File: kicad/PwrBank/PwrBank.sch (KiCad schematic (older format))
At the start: 6 parts

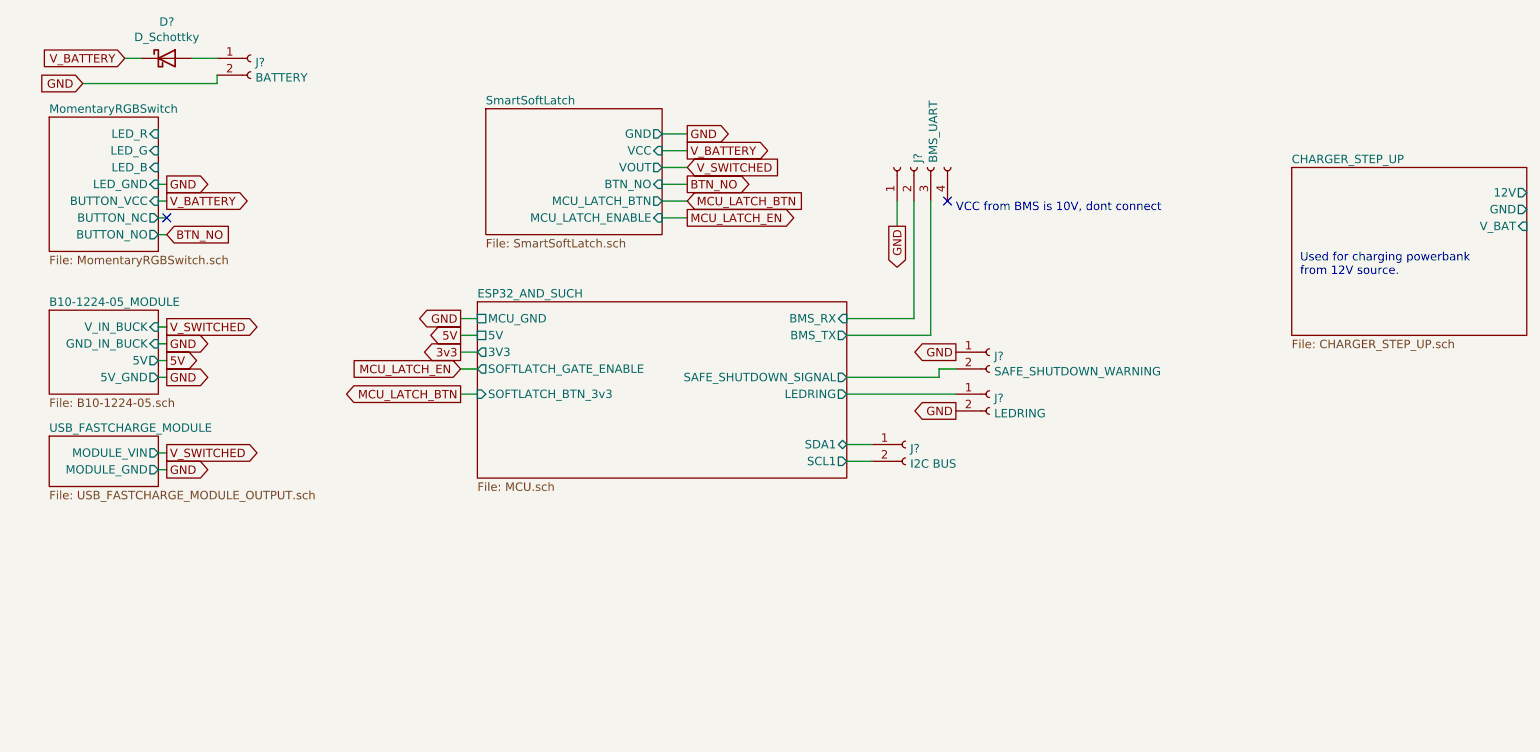
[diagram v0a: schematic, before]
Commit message: UPDATE KICAD SOURCEFILES
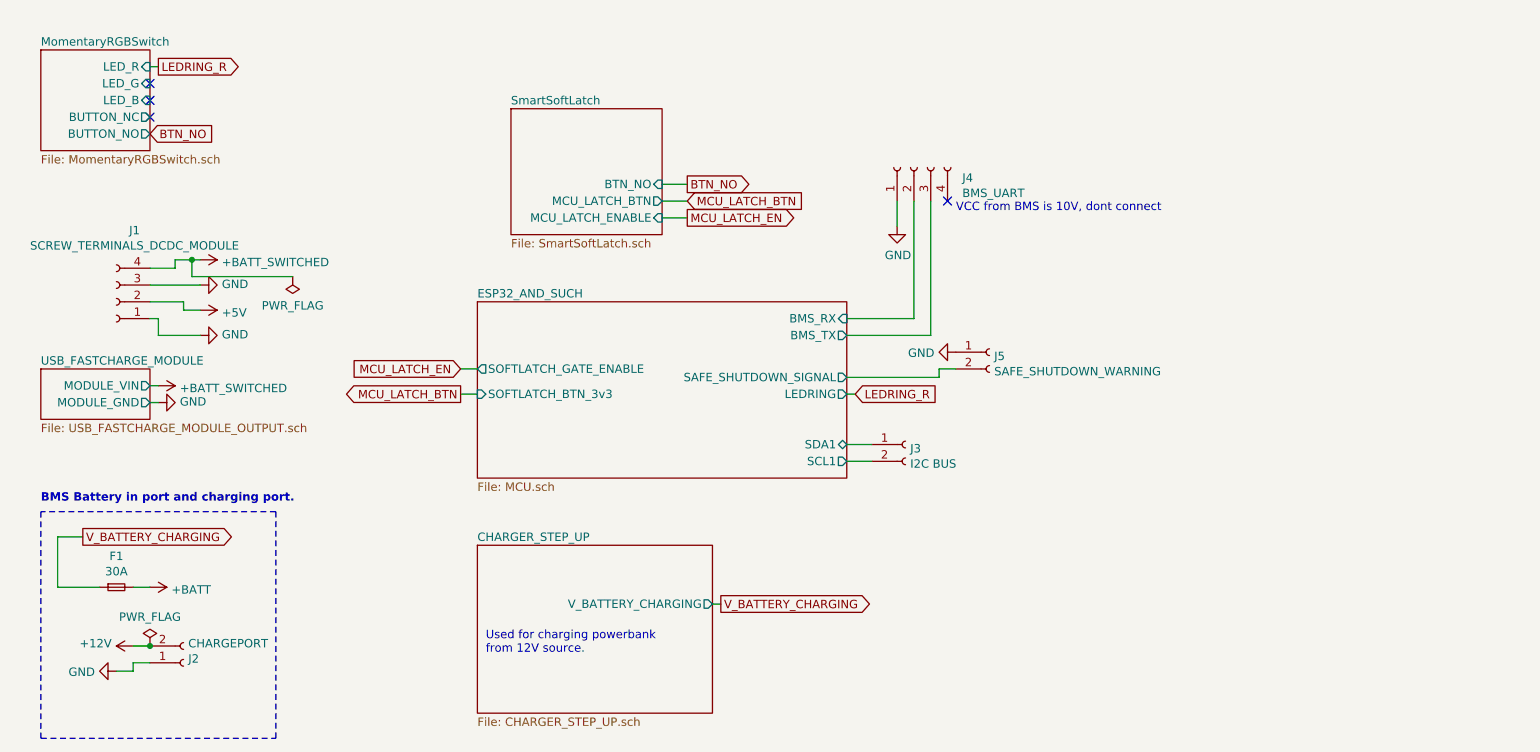
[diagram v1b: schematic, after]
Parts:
- removed D?: D_Schottky, symbol Device:D_Schottky
- removed J?: LEDRING, symbol Connector:Conn_01x02_Female
- removed J?: BATTERY, symbol Connector:Conn_01x02_Female
- added F1: 30A, Fuse:Fuseholder_Blade_Mini_Keystone_3568, symbol Device:Fuse_Small
- added J1: SCREW_TERMINALS_DCDC_MODULE, symbol Connector:Conn_01x04_Female
- added J2: CHARGEPORT, Connector_JST:JST_XH_B2B-XH-A_1x02_P2.50mm_Vertical, symbol Connector:Conn_01x02_Female
- J3, J5: renamed from J?; footprint (none) -> Connector_JST:JST_XH_B2B-XH-A_1x02_P2.50mm_Vertical
- J4: renamed from J?; footprint (none) -> Connector_JST:JST_XH_B4B-XH-A_1x04_P2.50mm_Vertical
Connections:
- net GND: now also J1.1 (Pin_1), J1.3 (Pin_3), J2.1 (Pin_1)
- new net +12V: J2.2 (Pin_2)
- new net +5V: J1.2 (Pin_2)
- new net +BATT: F1.2
- new net +BATT_SWITCHED: J1.4 (Pin_4)
- new net V_BATTERY_CHARGING: F1.1
- no-connect marks 2 -> 4
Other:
- note added: "BMS Battery in port and charging port."

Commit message: Kicad files update
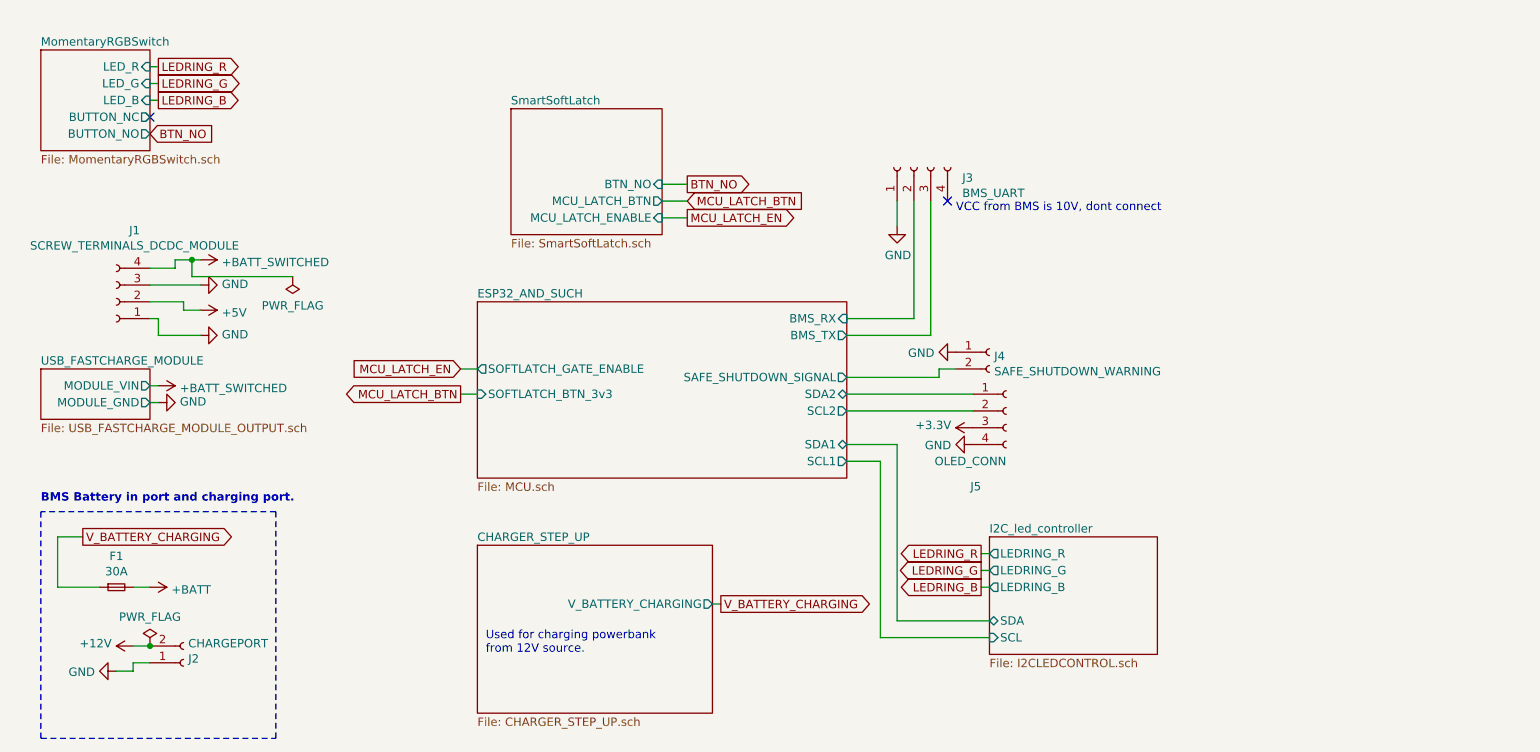
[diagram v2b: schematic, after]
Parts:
- removed J3: I2C BUS, Connector_JST:JST_XH_B2B-XH-A_1x02_P2.50mm_Vertical, symbol Connector:Conn_01x02_Female
- added J5: OLED_CONN, Connector_JST:JST_XH_B4B-XH-A_1x04_P2.50mm_Vertical, symbol Connector:Conn_01x04_Female
- renumbered J4 to J3, J5 to J4
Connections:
- net GND: now also J5.4 (Pin_4)
- new net +3V3: J5.3 (Pin_3)
- new net ESP32_AND_SUCH/SCL2: J5.2 (Pin_2)
- new net ESP32_AND_SUCH/SDA2: J5.1 (Pin_1)
- no-connect marks 4 -> 2
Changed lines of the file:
@@
 $Descr A4 11693 8268
 encoding utf-8
-Sheet 1 8
+Sheet 1 9
 Title "Powerbank BMS Additional Circuitry"
 Date "2021-07-11"
@@
 F3 "LED_G" I R 1250 900 50
 F4 "LED_B" I R 1250 1000 50
-F7 "BUTTON_NC" O R 1250 1100 50
-F8 "BUTTON_NO" O R 1250 1200 50
+F5 "BUTTON_NC" O R 1250 1100 50
+F6 "BUTTON_NO" O R 1250 1200 50
 $EndSheet
 NoConn ~ 1250 1100
@@
 F0 "SmartSoftLatch" 50
 F1 "SmartSoftLatch.sch" 50
-F3 "BTN_NO" I R 4300 1500 50
-F5 "MCU_LATCH_BTN" O R 4300 1600 50
-F6 "MCU_LATCH_ENABLE" I R 4300 1700 50
+F2 "BTN_NO" I R 4300 1500 50
+F3 "MCU_LATCH_BTN" O R 4300 1600 50
+F4 "MCU_LATCH_ENABLE" I R 4300 1700 50
 $EndSheet
 Text GLabel 4450 1500 2    50   Output ~ 0
@@
 F0 "CHARGER_STEP_UP" 50
 F1 "CHARGER_STEP_UP.sch" 50
-F3 "V_BATTERY_CHARGING" O R 4600 4000 50
+F2 "V_BATTERY_CHARGING" O R 4600 4000 50
 $EndSheet
 Text Notes 3250 4300 0    50   ~ 0
@@
 F4 "SAFE_SHUTDOWN_SIGNAL" O R 5400 2650 50
 F5 "SOFTLATCH_GATE_ENABLE" O L 3200 2600 50
-F6 "LEDRING" O R 5400 2750 50
-F7 "SDA1" B R 5400 3050 50
-F8 "SCL1" O R 5400 3150 50
-F9 "SOFTLATCH_BTN_3v3" I L 3200 2750 50
+F6 "SDA1" B R 5400 3050 50
+F7 "SCL1" O R 5400 3150 50
+F8 "SOFTLATCH_BTN_3v3" I L 3200 2750 50
+F9 "SCL2" O R 5400 2850 50
+F10 "SDA2" B R 5400 2750 50
 $EndSheet
 Text GLabel 3100 2600 0    50   Input ~ 0
@@
 Text GLabel 4450 1600 2    50   Input ~ 0
 MCU_LATCH_BTN
-$Comp
-L Connector:Conn_01x02_Female J3
-U 1 1 60F61784
-P 5750 3050
-F 0 "J3" H 5778 3026 50  0000 L CNN
-F 1 "I2C BUS" H 5778 2935 50  0000 L CNN
-F 2 "Connector_JST:JST_XH_B2B-XH-A_1x02_P2.50mm_Vertical" H 5750 3050 50  0001 C CNN
-F 3 "~" H 5750 3050 50  0001 C CNN
-	1    5750 3050
-	1    0    0    -1
-$EndComp
-Wire Wire Line
-	5400 3050 5550 3050
-Wire Wire Line
-	5550 3150 5400 3150
 Wire Wire Line
 	5400 2650 5950 2650
@@
 	5950 2600 6050 2600
 $Comp
-L Connector:Conn_01x04_Female J4
+L Connector:Conn_01x04_Female J3
 U 1 1 60F67167
 P 5800 1400
-F 0 "J4" V 5738 1112 50  0000 R CNN
+F 0 "J3" V 5738 1112 50  0000 R CNN
 F 1 "BMS_UART" V 5647 1112 50  0000 R CNN
 F 2 "Connector_JST:JST_XH_B4B-XH-A_1x04_P2.50mm_Vertical" H 5800 1400 50  0001 C CNN
@@
 Text Notes 600  3400 0    50   ~ 10
 BMS Battery in port and charging port.
-Text GLabel 5450 2750 2    50   Input ~ 0
-LEDRING_R
-Wire Wire Line
-	5450 2750 5400 2750
 Text GLabel 1300 800  2    50   Output ~ 0
 LEDRING_R
 Wire Wire Line
 	1300 800  1250 800
-NoConn ~ 1250 900
-NoConn ~ 1250 1000
 $Comp
 L power:+BATT #PWR03
@@
 $EndComp
 $Comp
-L Connector:Conn_01x02_Female J5
+L Connector:Conn_01x02_Female J4
 U 1 1 60F64EEF
 P 6250 2500
-F 0 "J5" H 6278 2476 50  0000 L CNN
+F 0 "J4" H 6278 2476 50  0000 L CNN
 F 1 "SAFE_SHUTDOWN_WARNING" H 6278 2385 50  0000 L CNN
 F 2 "Connector_JST:JST_XH_B2B-XH-A_1x02_P2.50mm_Vertical" H 6250 2500 50  0001 C CNN
@@
 	0    1    1    0
 $EndComp
+$Comp
+L Connector:Conn_01x04_Female J5
+U 1 1 60F9EBFE
+P 6350 2850
+F 0 "J5" H 6200 2400 50  0000 R CNN
+F 1 "OLED_CONN" H 6350 2550 50  0000 R CNN
+F 2 "Connector_JST:JST_XH_B4B-XH-A_1x04_P2.50mm_Vertical" H 6350 2850 50  0001 C CNN
+F 3 "https://www.jst-mfg.com/product/pdf/eng/eXH.pdf" H 6350 2850 50  0001 C CNN
+	1    6350 2850
+	1    0    0    -1
+$EndComp
+Wire Wire Line
+	5400 2750 6150 2750
+Wire Wire Line
+	5400 2850 6150 2850
+$Comp
+L power:+3.3V #PWR012
+U 1 1 60FA2045
+P 6150 2950
+F 0 "#PWR012" H 6150 2800 50  0001 C CNN
+F 1 "+3.3V" V 6165 3078 50  0000 L CNN
+F 2 "" H 6150 2950 50  0001 C CNN
+F 3 "" H 6150 2950 50  0001 C CNN
+	1    6150 2950
+	0    -1   -1   0
+$EndComp
+$Comp
+L power:GND #PWR013
+U 1 1 60FA2D4B
+P 6150 3050
+F 0 "#PWR013" H 6150 2800 50  0001 C CNN
+F 1 "GND" V 6155 2922 50  0000 R CNN
+F 2 "" H 6150 3050 50  0001 C CNN
+F 3 "" H 6150 3050 50  0001 C CNN
+	1    6150 3050
+	0    1    1    0
+$EndComp
+$Sheet
+S 6250 3600 1000 700
+U 60FA4163
+F0 "I2C_led_controller" 50
+F1 "I2CLEDCONTROL.sch" 50
+F2 "LEDRING_R" O L 6250 3700 50
+F3 "LEDRING_G" O L 6250 3800 50
+F4 "LEDRING_B" O L 6250 3900 50
+F5 "SDA" B L 6250 4100 50
+F6 "SCL" I L 6250 4200 50
+$EndSheet
+Wire Wire Line
+	5400 3150 5600 3150
+Wire Wire Line
+	5600 3150 5600 4200
+Wire Wire Line
+	5600 4200 6250 4200
+Wire Wire Line
+	5400 3050 5700 3050
+Wire Wire Line
+	5700 3050 5700 4100
+Wire Wire Line
+	5700 4100 6250 4100
+Text GLabel 6200 3700 0    50   Output ~ 0
+LEDRING_R
+Text GLabel 6200 3800 0    50   Output ~ 0
+LEDRING_G
+Text GLabel 6200 3900 0    50   Output ~ 0
+LEDRING_B
+Wire Wire Line
+	6200 3700 6250 3700
+Wire Wire Line
+	6200 3800 6250 3800
+Wire Wire Line
+	6200 3900 6250 3900
+Text GLabel 1300 900  2    50   Output ~ 0
+LEDRING_G
+Text GLabel 1300 1000 2    50   Output ~ 0
+LEDRING_B
+Wire Wire Line
+	1250 900  1300 900
+Wire Wire Line
+	1250 1000 1300 1000
 $EndSCHEMATC
